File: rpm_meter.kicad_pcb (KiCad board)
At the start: 2 copper layers, 153.8 x 95.2 mm, 123 parts, among them IC1 SN74LV1T34DCKR, IC6 TPS566247DRLR, J1 Conn_01x01_Socket, J2 Conn_2Rows-05Pins, J3 Conn_01x01_Socket, J4 Conn_01x01_Socket, J5 Conn_01x01_Socket, J6 Conn_01x01_Socket, J7 Conn_01x01_Socket, Q1 BC846, Q14 BC846, Q15 BC846, Q16 BC846, SW1 RotaryEncoder_Switch_MP, U1 M24C02-RMN, U2 STM32C031C6Tx, U3 74LVC1G123, U4 TLV1117-33, Y1 8

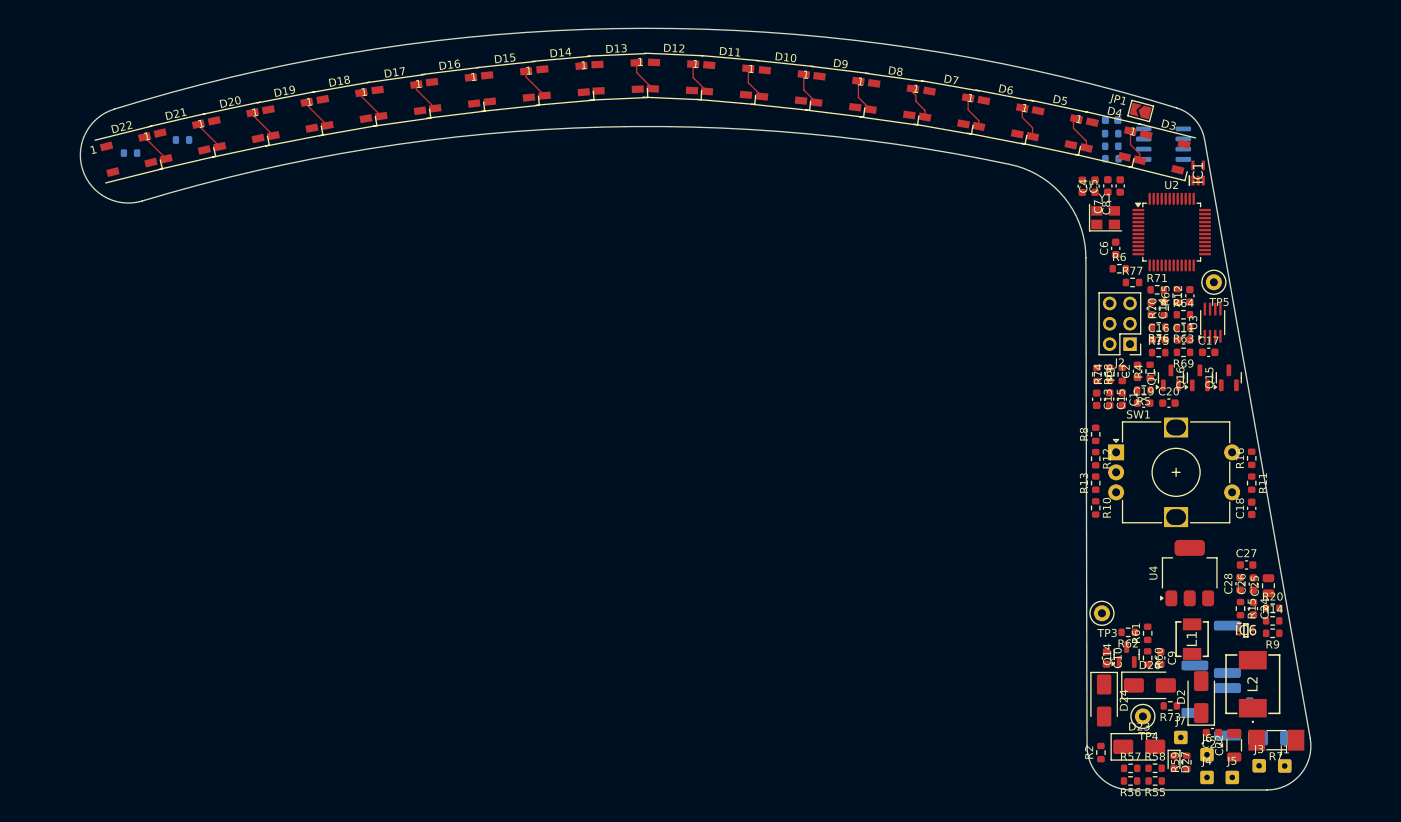
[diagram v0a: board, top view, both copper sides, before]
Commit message: 2.1
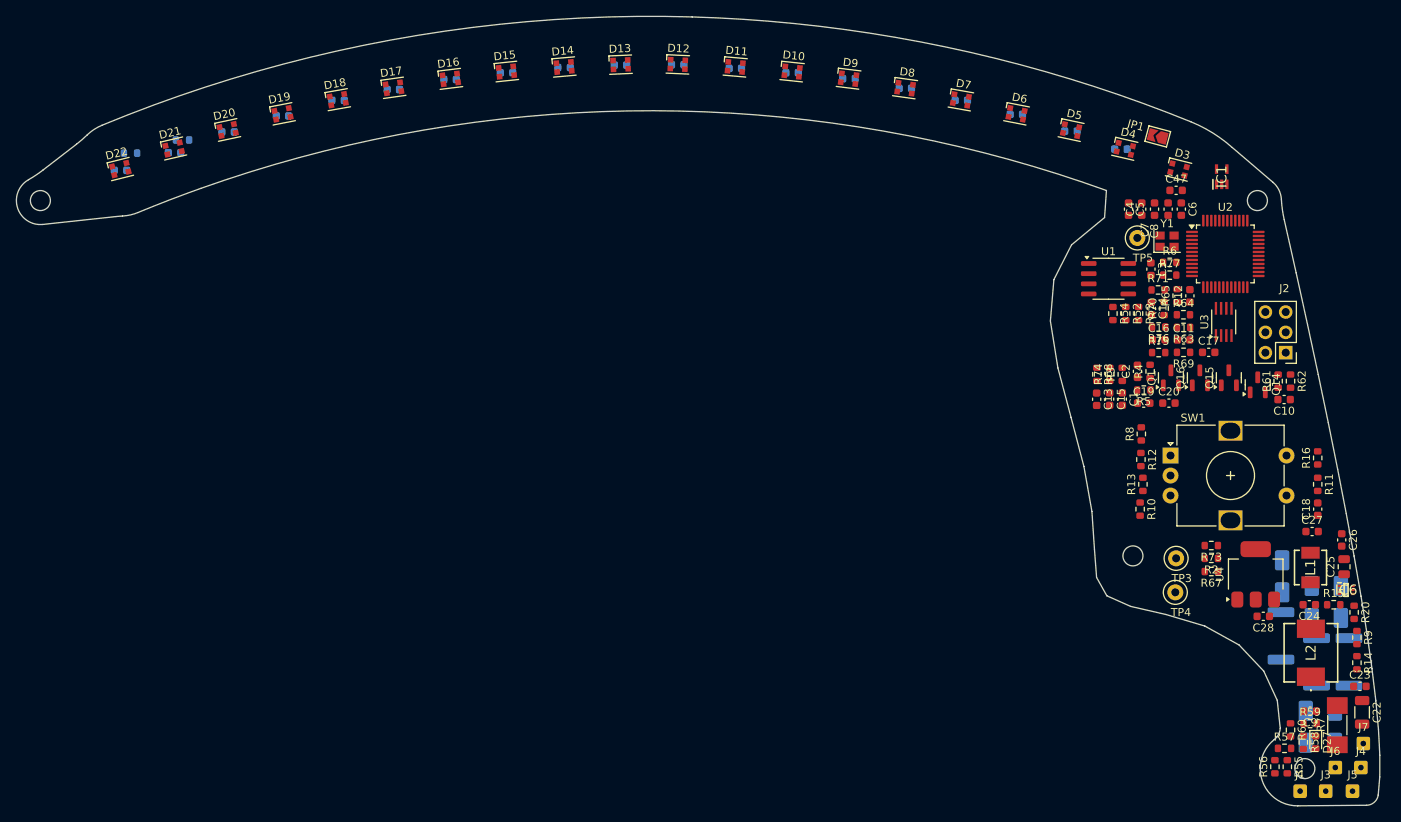
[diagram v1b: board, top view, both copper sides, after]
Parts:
- added C21: 100n, Capacitor_SMD:C_0603_1608Metric, B.Cu at (73.2, 47.4)
- added C29: 100n, Capacitor_SMD:C_0603_1608Metric, B.Cu at (100.3, 38.6)
- added C30: 100n, Capacitor_SMD:C_0603_1608Metric, B.Cu at (128.6, 34.5)
- added C31: 100n, Capacitor_SMD:C_0603_1608Metric, B.Cu at (135.7, 34.2)
- added C32: 100n, Capacitor_SMD:C_0603_1608Metric, B.Cu at (142.8, 34.2)
- added C33: 100n, Capacitor_SMD:C_0603_1608Metric, B.Cu at (79.9, 45.2)
- added C34: 100n, Capacitor_SMD:C_0603_1608Metric, B.Cu at (107.2, 37.3)
- added C35: 100n, Capacitor_SMD:C_0603_1608Metric, B.Cu at (157.1, 35.2)
- added C36: 100n, Capacitor_SMD:C_0603_1608Metric, B.Cu at (164.2, 36.0)
- added C37: 100n, Capacitor_SMD:C_0603_1608Metric, B.Cu at (150.0, 34.6)
- added C38: 100n, Capacitor_SMD:C_0603_1608Metric, B.Cu at (86.6, 42.6)
- added C39: 100n, Capacitor_SMD:C_0603_1608Metric, B.Cu at (114.3, 36.0)
- added C40: 100n, Capacitor_SMD:C_0603_1608Metric, B.Cu at (171.2, 37.1)
- added C41: 100n, Capacitor_SMD:C_0603_1608Metric, B.Cu at (178.2, 38.6)
- added C42: 100n, Capacitor_SMD:C_0603_1608Metric, B.Cu at (185.1, 40.4)
- added C43: 100n, Capacitor_SMD:C_0603_1608Metric, B.Cu at (93.4, 40.6)
- added C44: 100n, Capacitor_SMD:C_0603_1608Metric, B.Cu at (121.4, 35.2)
- added C45: 100n, Capacitor_SMD:C_0603_1608Metric, B.Cu at (191.9, 42.5)
- added C46: 100n, Capacitor_SMD:C_0603_1608Metric, B.Cu at (198.2, 44.8)
- added C47: 100n, Capacitor_SMD:C_0603_1608Metric, F.Cu at (205.1, 49.9)
- C3, R52, R53, R54, R67, U1: moved to F.Cu
- D10, D11, D12, D13, D14, D15, D16, D17, D18, D19, D20, D21, D22, D3, D4, D5, D6, D7, D8, D9: footprint LED_SMD:LED_WS2812B_PLCC4_5.0x5.0mm_P3.2mm -> Library_local:LED_WS2812B-2020_PLCC4_2.0x2.0mm
- D2, D23, D24, D26: moved to B.Cu
- Y1: footprint Crystal:Crystal_SMD_3225-4Pin_3.2x2.5mm -> Crystal:Crystal_SMD_2520-4Pin_2.5x2.0mm
- moved C10 39.2 mm to (218.6, 76.0), turned to 180 degrees
- moved Q14 37.5 mm to (215.3, 74.2)
- moved R62 37.4 mm to (219.4, 73.8), turned to -90 degrees
- moved R61 35.5 mm to (217.8, 73.8)
- moved D24 28.7 mm to (222.1, 101.3)
- moved R2 27.9 mm to (209.5, 95.9), turned to 180 degrees
- moved D26 26.1 mm to (225.7, 101.3), turned to -90 degrees
- moved J7 22.8 mm to (228.5, 119.0)
- moved R54 22.5 mm to (197.2, 65.3), turned to -90 degrees
- moved R53 21.2 mm to (200.4, 65.3), turned to -90 degrees
- moved D23 21.0 mm to (221.3, 117.0), turned to -90 degrees
- moved R73 20.7 mm to (209.5, 94.3)
- moved D25 20.3 mm to (218.3, 98.2), turned to -90 degrees
- moved R60 20.0 mm to (219.4, 117.3)
- moved C9 19.8 mm to (221.8, 115.0), turned to 180 degrees
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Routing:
- net Net-(D4-DOUT): track 4.45 -> 0.00 mm
- net Net-(D10-DOUT): track 4.21 -> 0.00 mm
- net Net-(D8-DOUT): track 4.19 -> 0.00 mm
- net Net-(D10-DIN): track 4.16 -> 0.00 mm
- net Net-(D7-DOUT): track 4.15 -> 0.00 mm
- net Net-(D3-DOUT): track 4.13 -> 0.00 mm
- net Net-(D11-DOUT): track 4.13 -> 0.00 mm
- net Net-(D6-DOUT): track 4.12 -> 0.00 mm
- net Net-(D5-DOUT): track 4.11 -> 0.00 mm
- net Net-(D12-DOUT): track 4.09 -> 0.00 mm
- net Net-(D14-DOUT): track 4.00 -> 0.00 mm
- net Net-(D17-DOUT): track 3.98 -> 0.00 mm
- net Net-(D18-DOUT): track 3.96 -> 0.00 mm
- net Net-(D19-DOUT): track 3.95 -> 0.00 mm
- net Net-(D16-DOUT): track 3.95 -> 0.00 mm
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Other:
- board size 153.8 x 95.2 mm -> 170.4 x 98.7 mm
